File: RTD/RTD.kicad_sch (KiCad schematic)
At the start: 48 parts, among them SW1 SW_SPDT, U1 THVD1420D, U2 STM32F103C8Tx

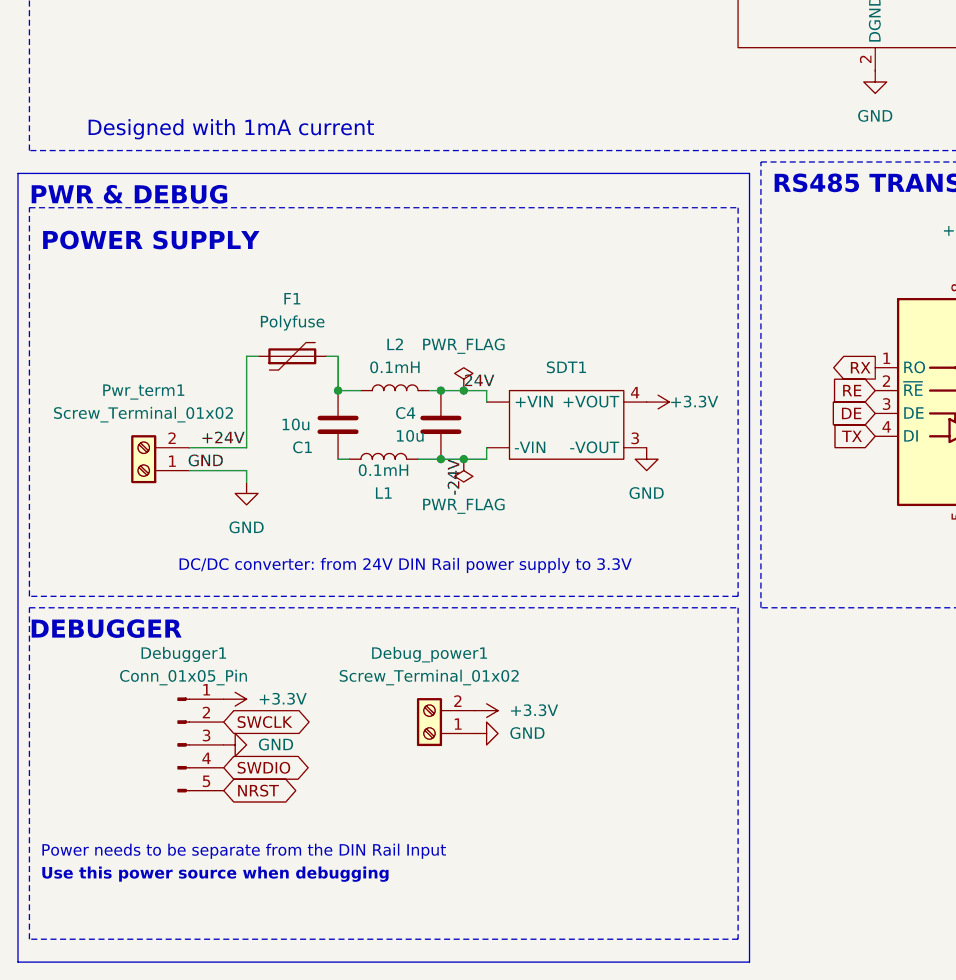
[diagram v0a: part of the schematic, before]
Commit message: light refactor
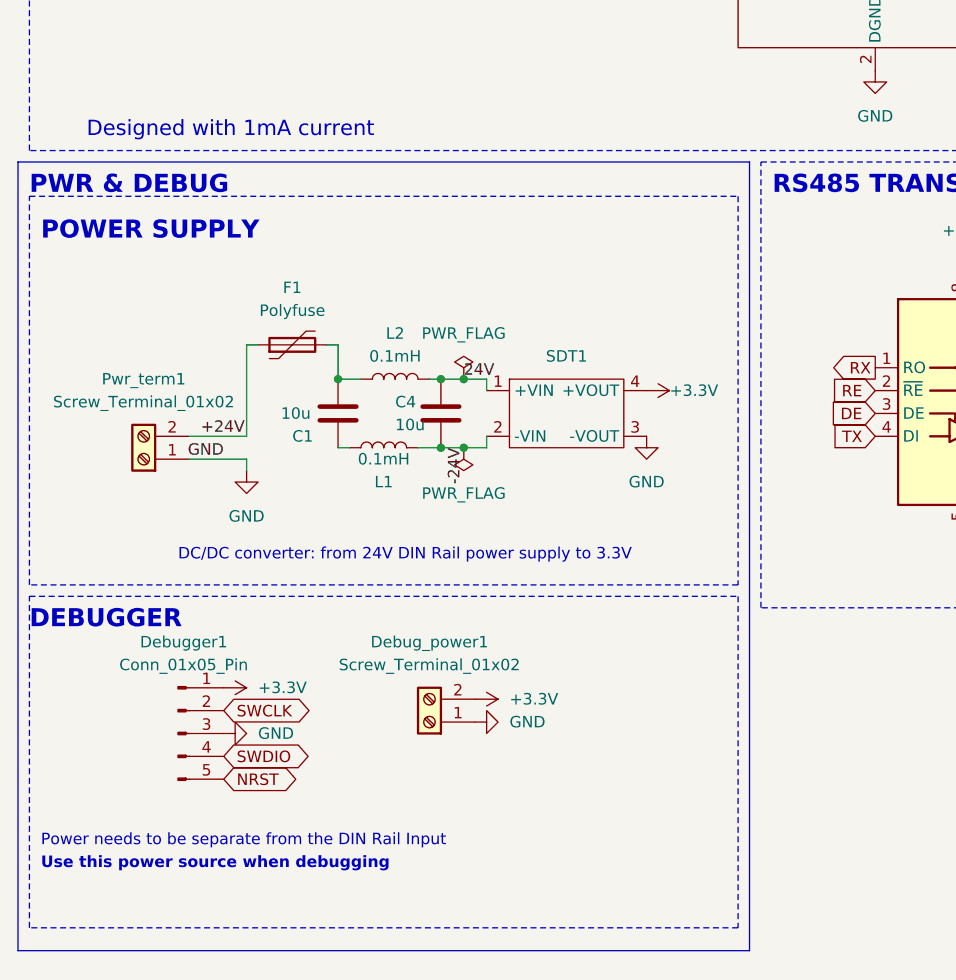
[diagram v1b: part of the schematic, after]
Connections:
- net -24V: now also SDT1.2 (-VIN); no longer SDT1. (-VIN)
- net 24V: now also SDT1.1 (+VIN); no longer SDT1. (-VIN)
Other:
- moved on the sheet: C1, C4, Debug_power1, Debugger1, F1, L1, L2, Pwr_term1
